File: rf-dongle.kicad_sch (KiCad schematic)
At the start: 35 parts, among them J1 USB_A, J3 TC2030, SW1 SW_Push, SW2 SW_Push, U1 nRF52840-QIXX, X1 32MHz, X2 32.768kHz

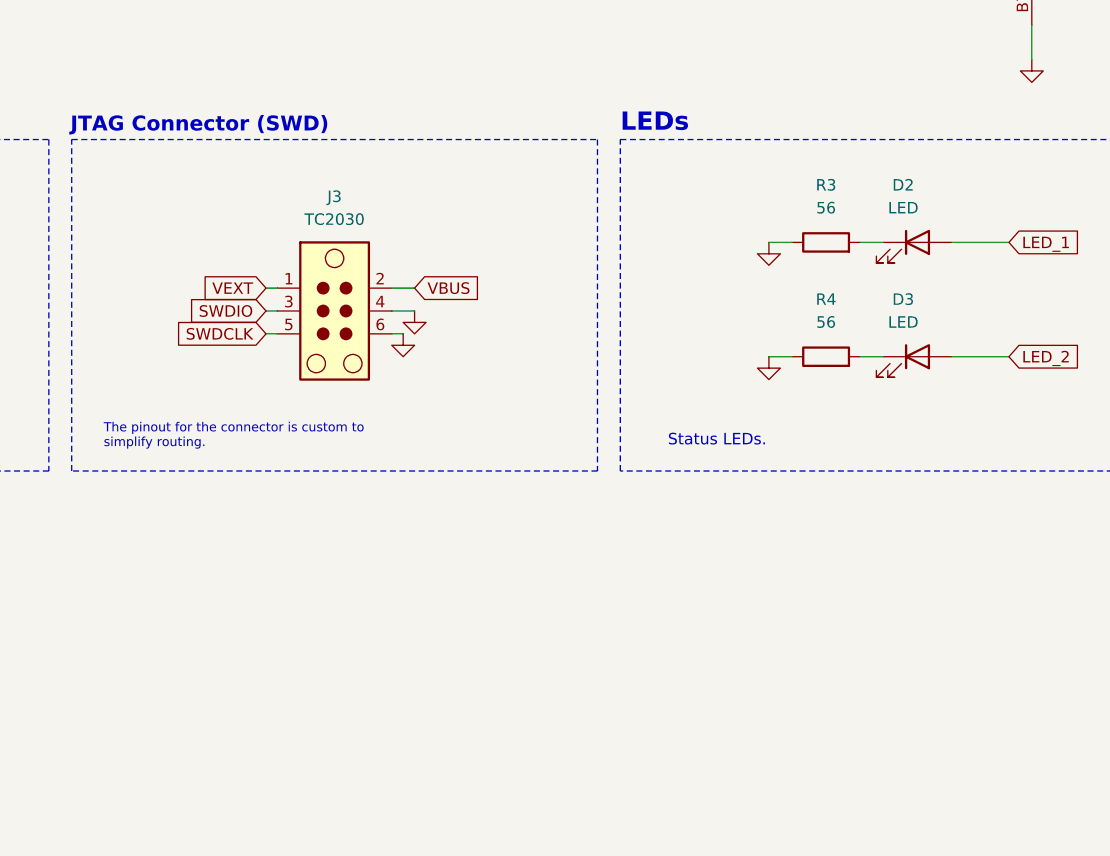
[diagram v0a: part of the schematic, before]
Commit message: before new programming pins
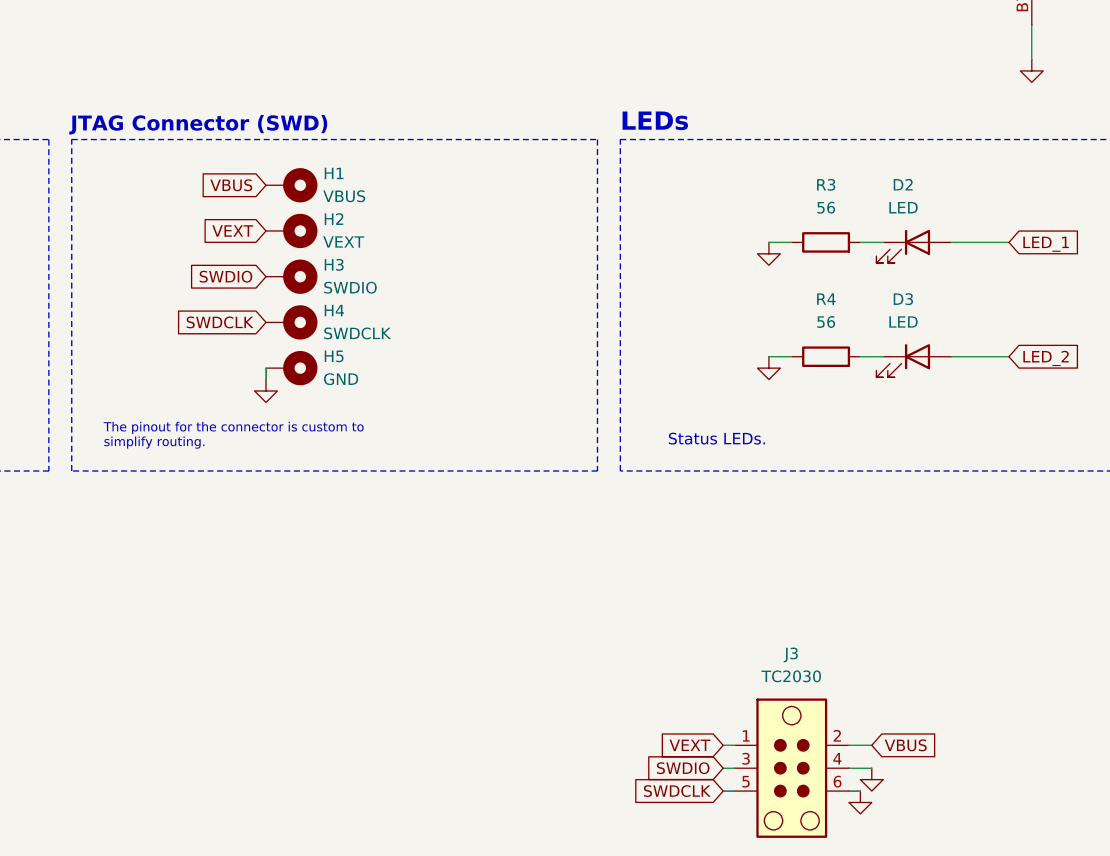
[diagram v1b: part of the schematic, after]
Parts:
- added H1: VBUS, TestPoint:TestPoint_THTPad_D1.0mm_Drill0.5mm, symbol Mechanical:MountingHole_Pad
- added H2: VEXT, TestPoint:TestPoint_THTPad_D1.0mm_Drill0.5mm, symbol Mechanical:MountingHole_Pad
- added H3: SWDIO, TestPoint:TestPoint_THTPad_D1.0mm_Drill0.5mm, symbol Mechanical:MountingHole_Pad
- added H4: SWDCLK, TestPoint:TestPoint_THTPad_D1.0mm_Drill0.5mm, symbol Mechanical:MountingHole_Pad
- added H5: GND, TestPoint:TestPoint_THTPad_D1.0mm_Drill0.5mm, symbol Mechanical:MountingHole_Pad
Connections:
- net GND: now also H5.1
- net SWDCLK: now also H4.1
- net SWDIO: now also H3.1
- net VBUS: now also H1.1
- net VEXT: now also H2.1
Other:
- moved on the sheet: J3
